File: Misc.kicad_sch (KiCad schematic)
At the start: 14 parts, among them J1 BM04B-SURS-TFLFSN, J501 Conn_01x04, U2 SN65HVD232QDRQ1

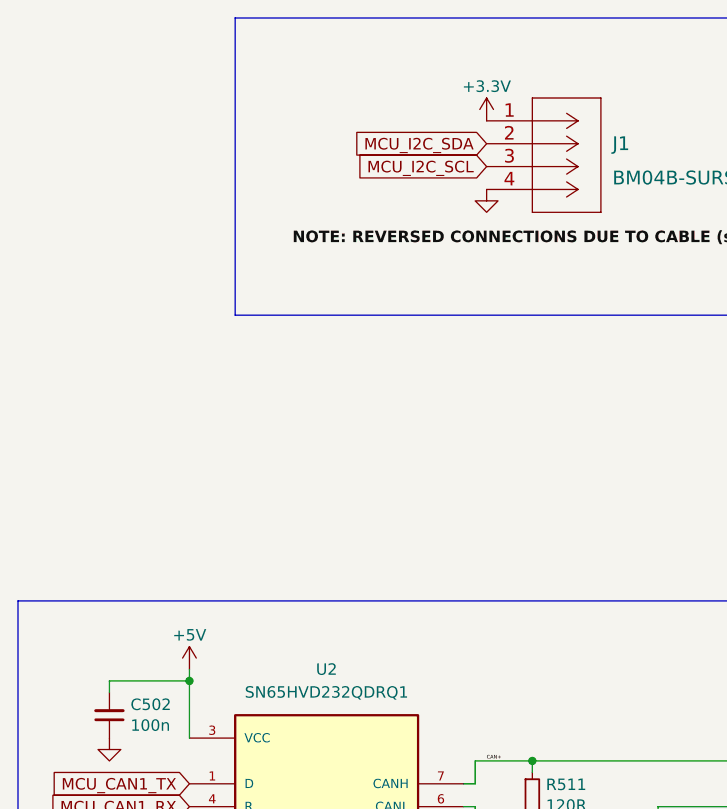
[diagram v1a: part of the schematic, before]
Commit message: more changes!
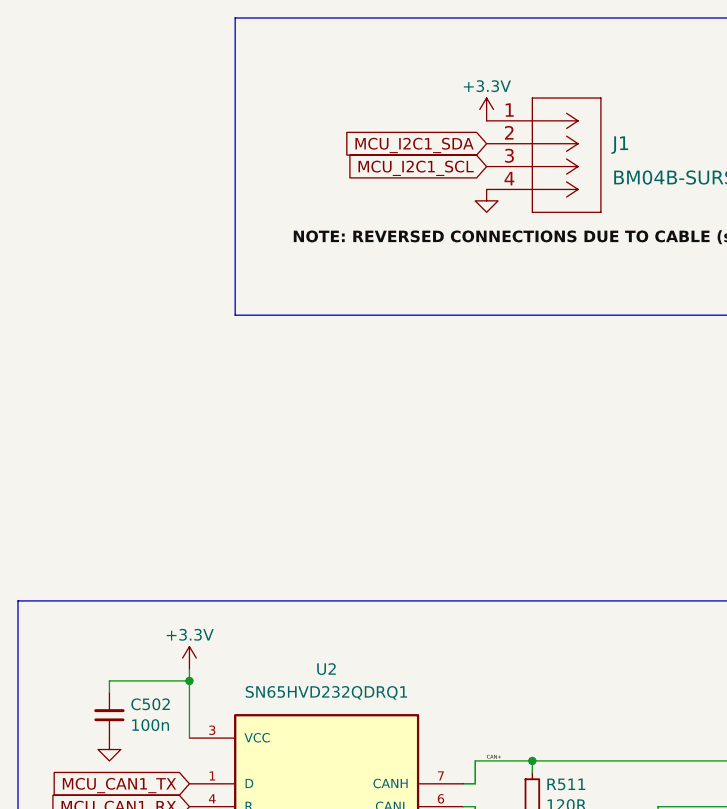
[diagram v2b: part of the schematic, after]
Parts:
- J1: footprint CONN_BM04B-SURS-TF_JST -> BM04B:BM04B-SURS-TFLFSN
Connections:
- net +5V is gone; now on net +3V3: C502.2, U2.3 (VCC)
- net MCU_I2C_SCL renamed MCU_I2C1_SCL
- net MCU_I2C_SDA renamed MCU_I2C1_SDA
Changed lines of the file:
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@@
     )
   )
-  (global_label "MCU_I2C_SCL" (shape input) (at 137.16 55.88 180) (fields_autoplaced)
+  (global_label "MCU_I2C1_SCL" (shape input) (at 137.16 55.88 180) (fields_autoplaced)
     (effects (font (size 1.27 1.27)) (justify right))
-    (property "Intersheet References" "${INTERSHEET_REFS}" (id 0) (at 122.2568 55.8006 0)
+    (property "Intersheet References" "${INTERSHEET_REFS}" (id 0) (at 121.0472 55.8006 0)
       (effects (font (size 1.27 1.27)) (justify right) hide)
     )
@@
     )
   )
-  (global_label "MCU_I2C_SDA" (shape input) (at 137.16 53.34 180) (fields_autoplaced)
+  (global_label "MCU_I2C1_SDA" (shape input) (at 137.16 53.34 180) (fields_autoplaced)
     (effects (font (size 1.27 1.27)) (justify right))
-    (property "Intersheet References" "${INTERSHEET_REFS}" (id 0) (at 122.1963 53.2606 0)
+    (property "Intersheet References" "${INTERSHEET_REFS}" (id 0) (at 120.9868 53.2606 0)
       (effects (font (size 1.27 1.27)) (justify right) hide)
     )
@@
     (pin "1")
     (pin "2")
-  )
-  (symbol (lib_id "power:+5V") (at 104.14 111.76 0) (unit 1)
-    (in_bom yes) (on_board yes)
-    (property "Reference" "#PWR051" (id 0) (at 104.14 115.57 0)
-      (effects (font (size 1.27 1.27)) hide)
-    )
-    (property "Value" "+5V" (id 1) (at 104.14 107.95 0))
-    (property "Footprint" "" (id 2) (at 104.14 111.76 0)
-      (effects (font (size 1.27 1.27)) hide)
-    )
-    (property "Datasheet" "" (id 3) (at 104.14 111.76 0)
-      (effects (font (size 1.27 1.27)) hide)
-    )
-    (pin "1")
   )
   (symbol (lib_id "Mechanical:MountingHole_Pad") (at 100.33 177.8 270) (unit 1)
@@
       (effects (font (size 1.524 1.524)) (justify left))
     )
-    (property "Footprint" "CONN_BM04B-SURS-TF_JST" (id 2) (at 147.32 57.404 0)
+    (property "Footprint" "BM04B:BM04B-SURS-TFLFSN" (id 2) (at 147.32 57.404 0)
       (effects (font (size 1.524 1.524)) hide)
     )
@@
     (pin "4")
   )
+  (symbol (lib_id "BluePhil-rescue:+3.3V-power") (at 104.14 111.76 0) (unit 1)
+    (in_bom yes) (on_board yes)
+    (property "Reference" "#PWR?" (id 0) (at 104.14 115.57 0)
+      (effects (font (size 1.27 1.27)) hide)
+    )
+    (property "Value" "+3.3V" (id 1) (at 104.14 107.95 0))
+    (property "Footprint" "" (id 2) (at 104.14 111.76 0)
+      (effects (font (size 1.27 1.27)) hide)
+    )
+    (property "Datasheet" "" (id 3) (at 104.14 111.76 0)
+      (effects (font (size 1.27 1.27)) hide)
+    )
+    (pin "1")
+  )
   (symbol (lib_id "power:GND") (at 137.16 58.42 0) (unit 1)

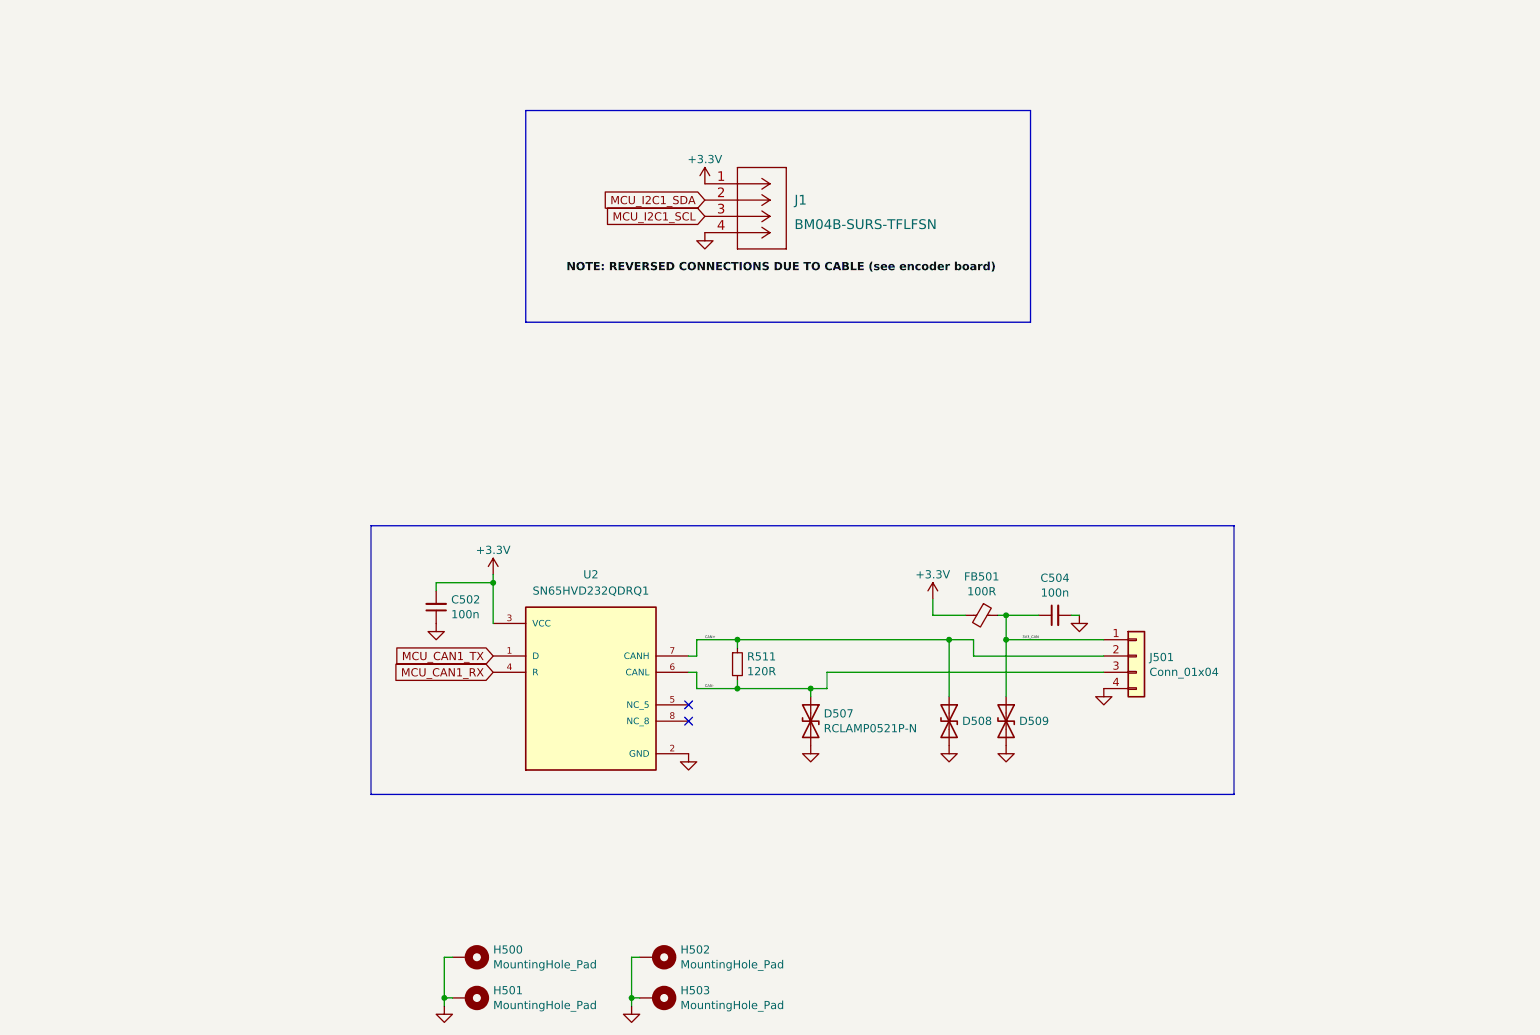
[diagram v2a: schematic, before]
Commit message: more progress
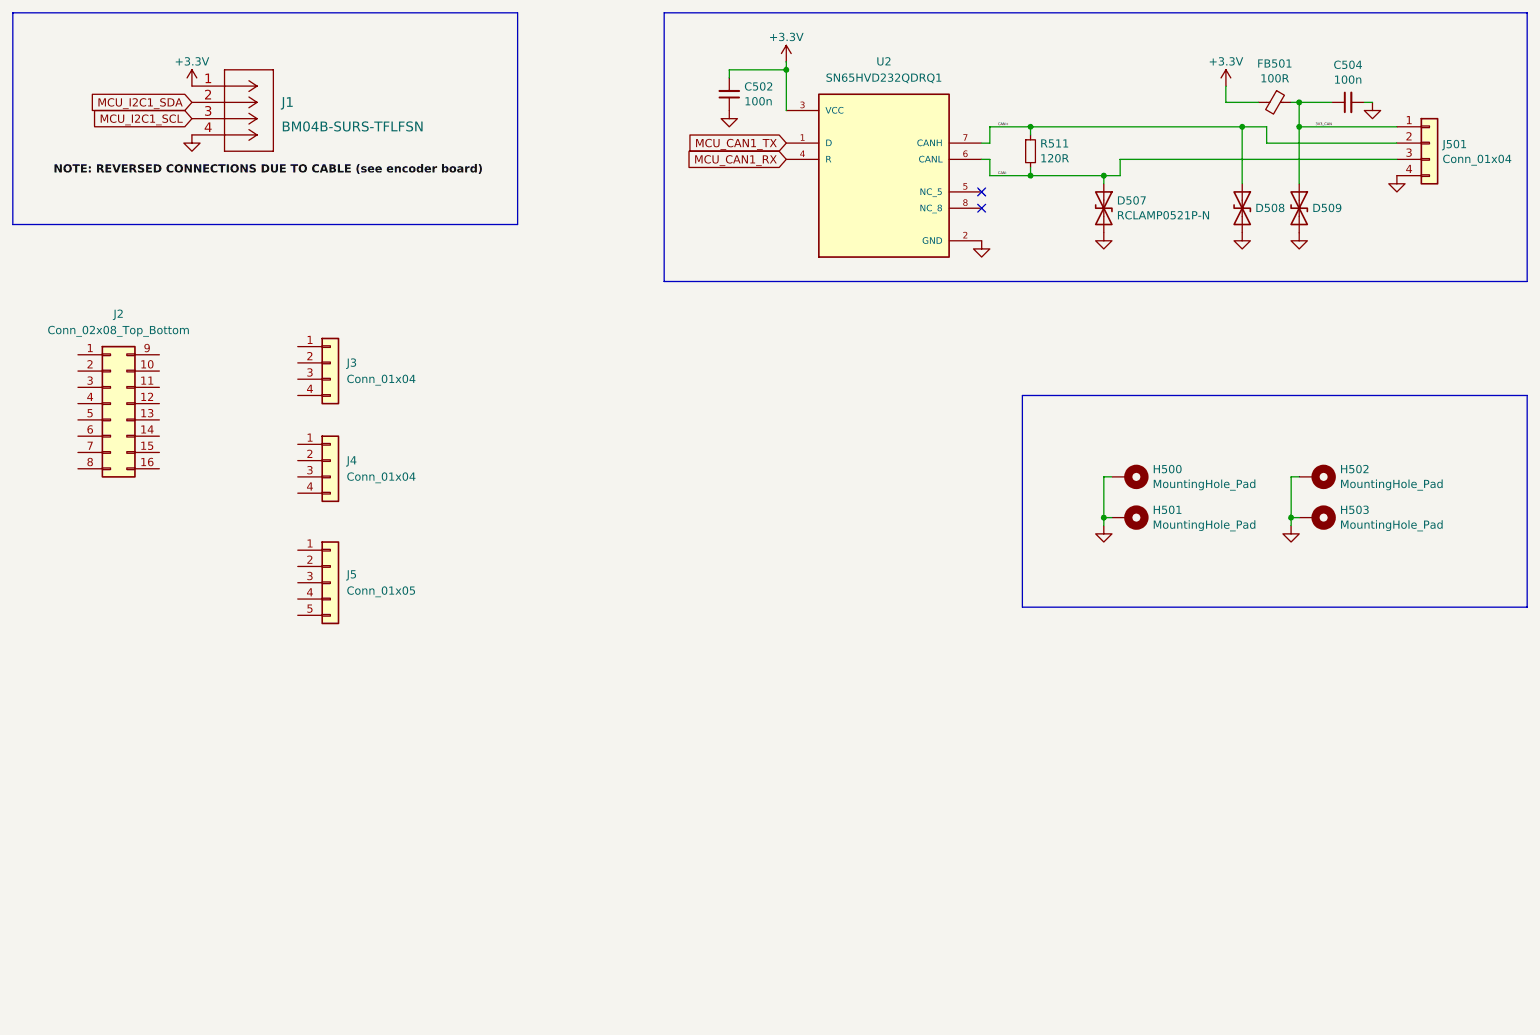
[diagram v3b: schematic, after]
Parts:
- added J2: Conn_02x08_Top_Bottom, Connector_PinSocket_2.54mm:PinSocket_2x08_P2.54mm_Vertical, symbol Connector_Generic:Conn_02x08_Top_Bottom
- added J3, J4: Conn_01x04, Connector_PinSocket_2.54mm:PinSocket_1x04_P2.54mm_Vertical, symbol Connector_Generic:Conn_01x04
- added J5: Conn_01x05, Connector_PinSocket_2.54mm:PinSocket_1x05_P2.54mm_Vertical, symbol Connector_Generic:Conn_01x05
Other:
- moved on the sheet: C502, C504, D507, D508, D509, FB501, H500, H501, H502, H503, J1, J501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
